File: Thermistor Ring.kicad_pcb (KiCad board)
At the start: 2 copper layers, 48.3 x 48.3 mm, 15 parts, among them J1 Conn_01x04_Socket, U2 MCP9808T-E/MC, U3 MCP9808T-E/MC, U4 MCP9808T-E/MC, U5 MCP9808T-E/MC, U6 MCP9808T-E/MC, U7 MCP9808T-E/MC

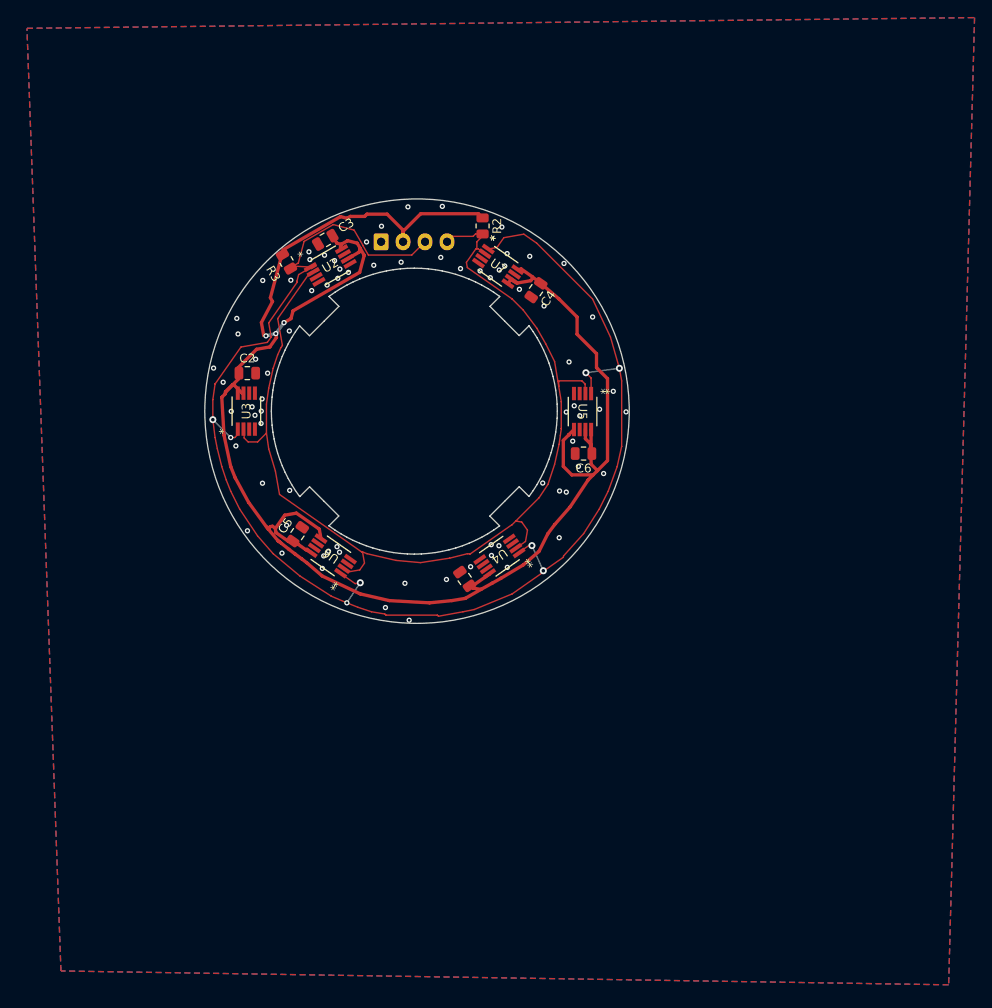
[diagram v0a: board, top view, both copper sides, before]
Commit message: Ouptut adjustments
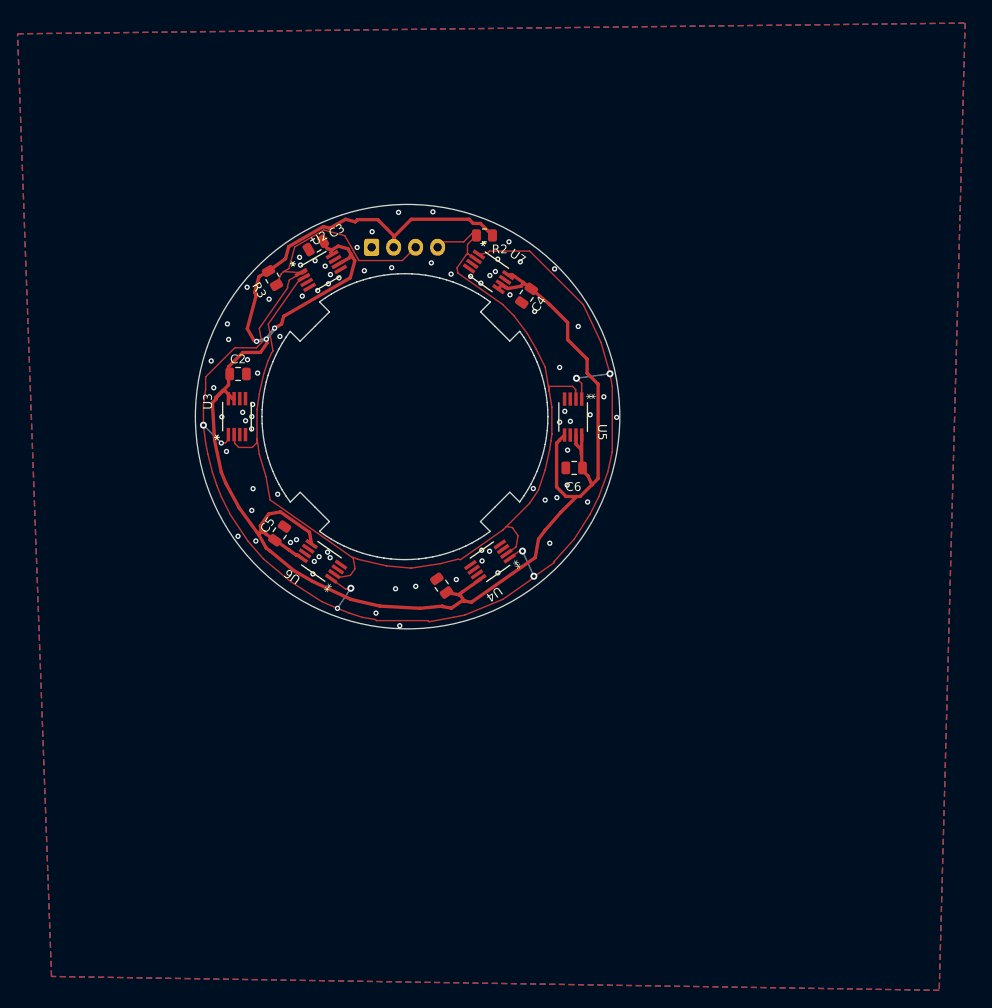
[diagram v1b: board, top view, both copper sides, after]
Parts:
- U2, U3, U4, U5, U6, U7: footprint MCP9808-E/MS:MSOP8_MC_MCH -> MCP9808-E/MS:MSOP8_MC_MCH_SMALL_PADS
- moved C1 2.72 mm to (77.9, 76.2)
- moved R3 2.46 mm to (58.7, 41.2)
- moved C5 2.02 mm to (59.5, 70.2)
- moved C6 1.95 mm to (93.0, 62.8)
- moved U6 1.24 mm to (64.2, 73.4)
- moved U4 1.24 mm to (83.4, 73.5)
- moved C3 1.24 mm to (63.6, 37.5)
- moved U3 1.24 mm to (54.6, 57.0)
- moved C4 1.24 mm to (87.5, 43.2)
- moved U7 1.24 mm to (83.2, 40.5)
- moved J1 1.24 mm to (69.9, 37.7)
- moved U2 1.24 mm to (64.2, 40.4)
- moved U5 1.24 mm to (92.8, 57.0)
- moved R2 1.10 mm to (82.8, 36.4), turned to 180 degrees
- moved C2 1.06 mm to (54.7, 52.1)
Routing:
- net /Power 3.3-5V: track 204.1 -> 213.8 mm
- net /SCL: track 123.0 -> 124.4 mm
- net /SDA: track 169.3 -> 170.2 mm
- net GND: vias 77 -> 79
